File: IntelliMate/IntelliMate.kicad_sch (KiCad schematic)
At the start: 61 parts, among them IC1 UDN2982LW, IC2 UDN2982LW, J1 Conn_01x03_Socket, Q1 Q_NPN_Darlington_BCE, Q10 Q_NMOS_GDS, Q11 Q_NMOS_GDS, Q12 Q_NMOS_GDS, Q13 Q_NMOS_GDS, Q14 Q_NMOS_GDS, Q15 Q_NMOS_GDS, Q16 Q_NMOS_GDS, Q2 Q_PNP_Darlington_BCE, Q3 Q_PNP_Darlington_BCE, Q4 Q_PNP_Darlington_BCE, Q5 Q_PNP_Darlington_BCE, Q6 Q_PNP_Darlington_BCE, Q7 Q_PNP_Darlington_BCE, Q8 Q_NMOS_GDS, Q9 Q_NMOS_GDS, U1 LM723_DIP14, U2 ULN2803A

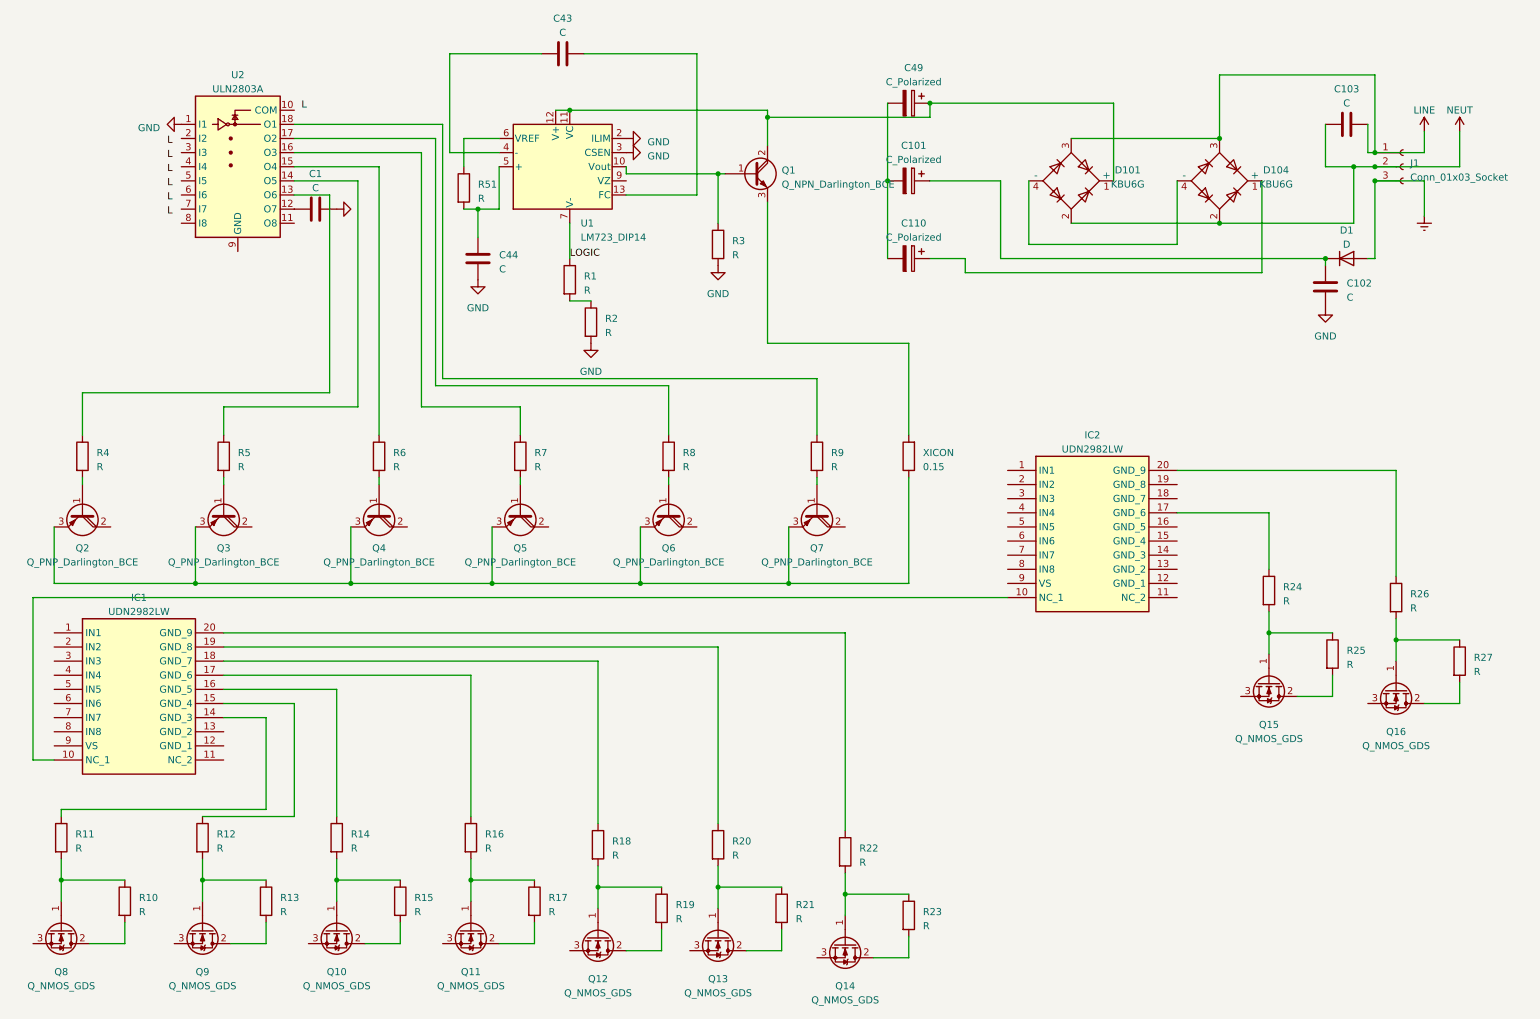
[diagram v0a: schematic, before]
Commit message: added multi pages
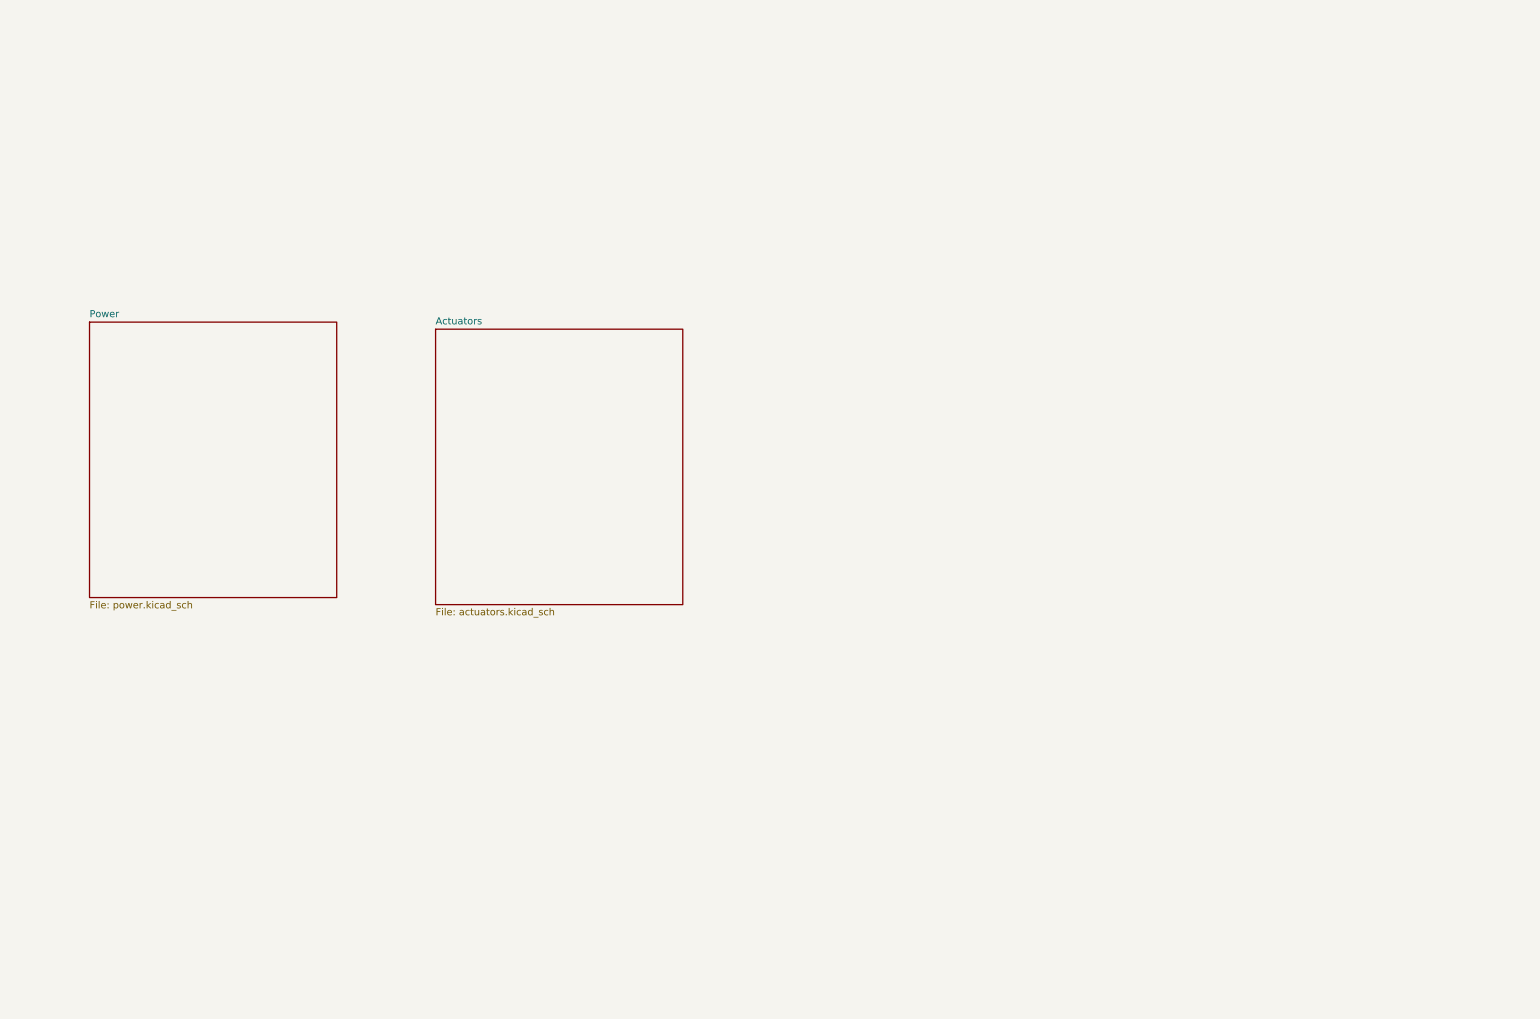
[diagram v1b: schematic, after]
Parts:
- removed C1, C102, C103, C43, C44: C, symbol Device:C
- removed C101, C110, C49: C_Polarized, symbol Device:C_Polarized
- removed D1: D, symbol Device:D
- removed D101, D104: KBU6G, Diode_THT:Diode_Bridge_Vishay_KBU, symbol Diode_Bridge:KBU6G
- removed IC1, IC2: UDN2982LW, SOIC127P1030X265-20N, symbol IntelliMate_Symbols:UDN2982LW
- removed J1: Conn_01x03_Socket, symbol Connector:Conn_01x03_Socket
- removed Q1: Q_NPN_Darlington_BCE, symbol Device:Q_NPN_Darlington_BCE
- removed Q10, Q11, Q12, Q13, Q14, Q15, Q16, Q8, Q9: Q_NMOS_GDS, symbol Device:Q_NMOS_GDS
- removed Q2, Q3, Q4, Q5, Q6, Q7: Q_PNP_Darlington_BCE, symbol Device:Q_PNP_Darlington_BCE
- removed R1, R10, R11, R12, R13, R14, R15, R16, R17, R18, R19, R2, R20, R21, R22, R23, R24, R25, R26, R27, R3, R4, R5, R51, R6, R7, R8, R9: R, symbol Device:R
- removed U1: LM723_DIP14, Package_DIP:DIP-14_W7.62mm, symbol Regulator_Linear:LM723_DIP14
- removed U2: ULN2803A, symbol Transistor_Array:ULN2803A
- removed XICON: 0.15, symbol Device:R
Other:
- added sheet Actuators (actuators.kicad_sch)
- added sheet Power (power.kicad_sch)
